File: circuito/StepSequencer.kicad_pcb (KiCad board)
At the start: 2 copper layers, 147.8 x 117.1 mm, 81 parts, among them P1 BEAGLEBONE_BLACK, SW0 SW_PUSH, SW1 SW_PUSH, SW10 SW_PUSH, SW11 SW_PUSH, SW12 SW_PUSH, SW13 SW_PUSH, SW14 SW_PUSH, SW15 SW_PUSH, SW2 SW_PUSH, SW3 SW_PUSH, SW4 SW_PUSH, SW5 SW_PUSH, SW6 SW_PUSH, SW7 SW_PUSH, SW8 SW_PUSH, SW9 SW_PUSH

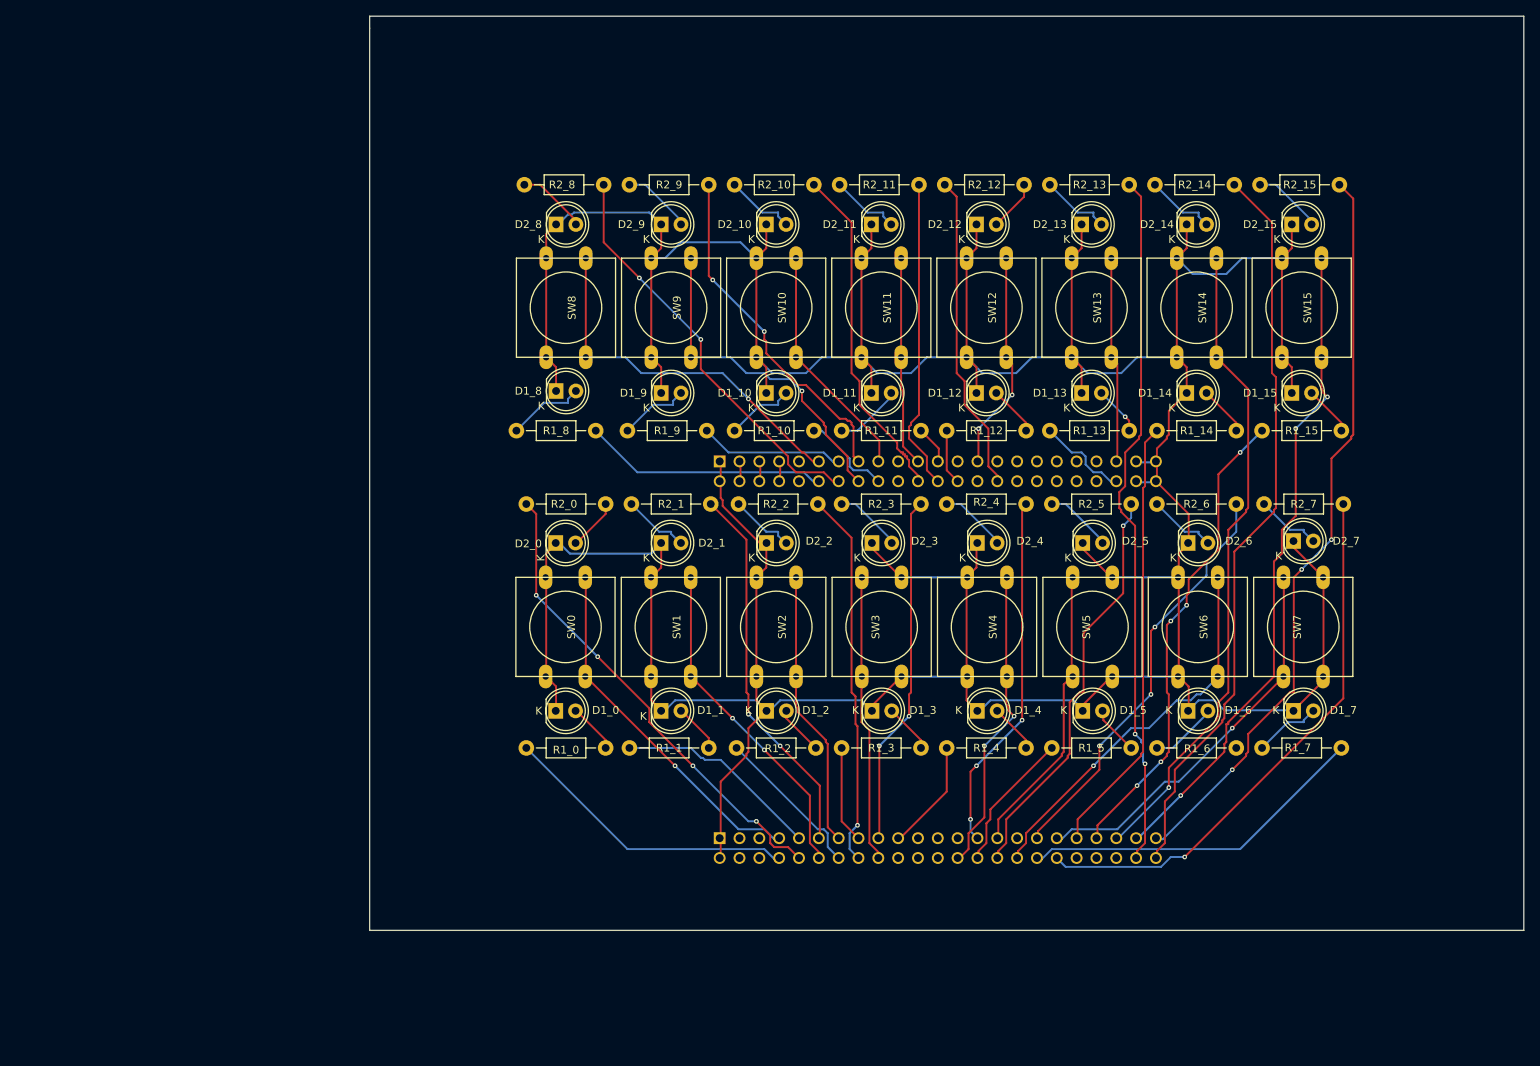
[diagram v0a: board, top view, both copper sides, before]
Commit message: PCB Casi listo
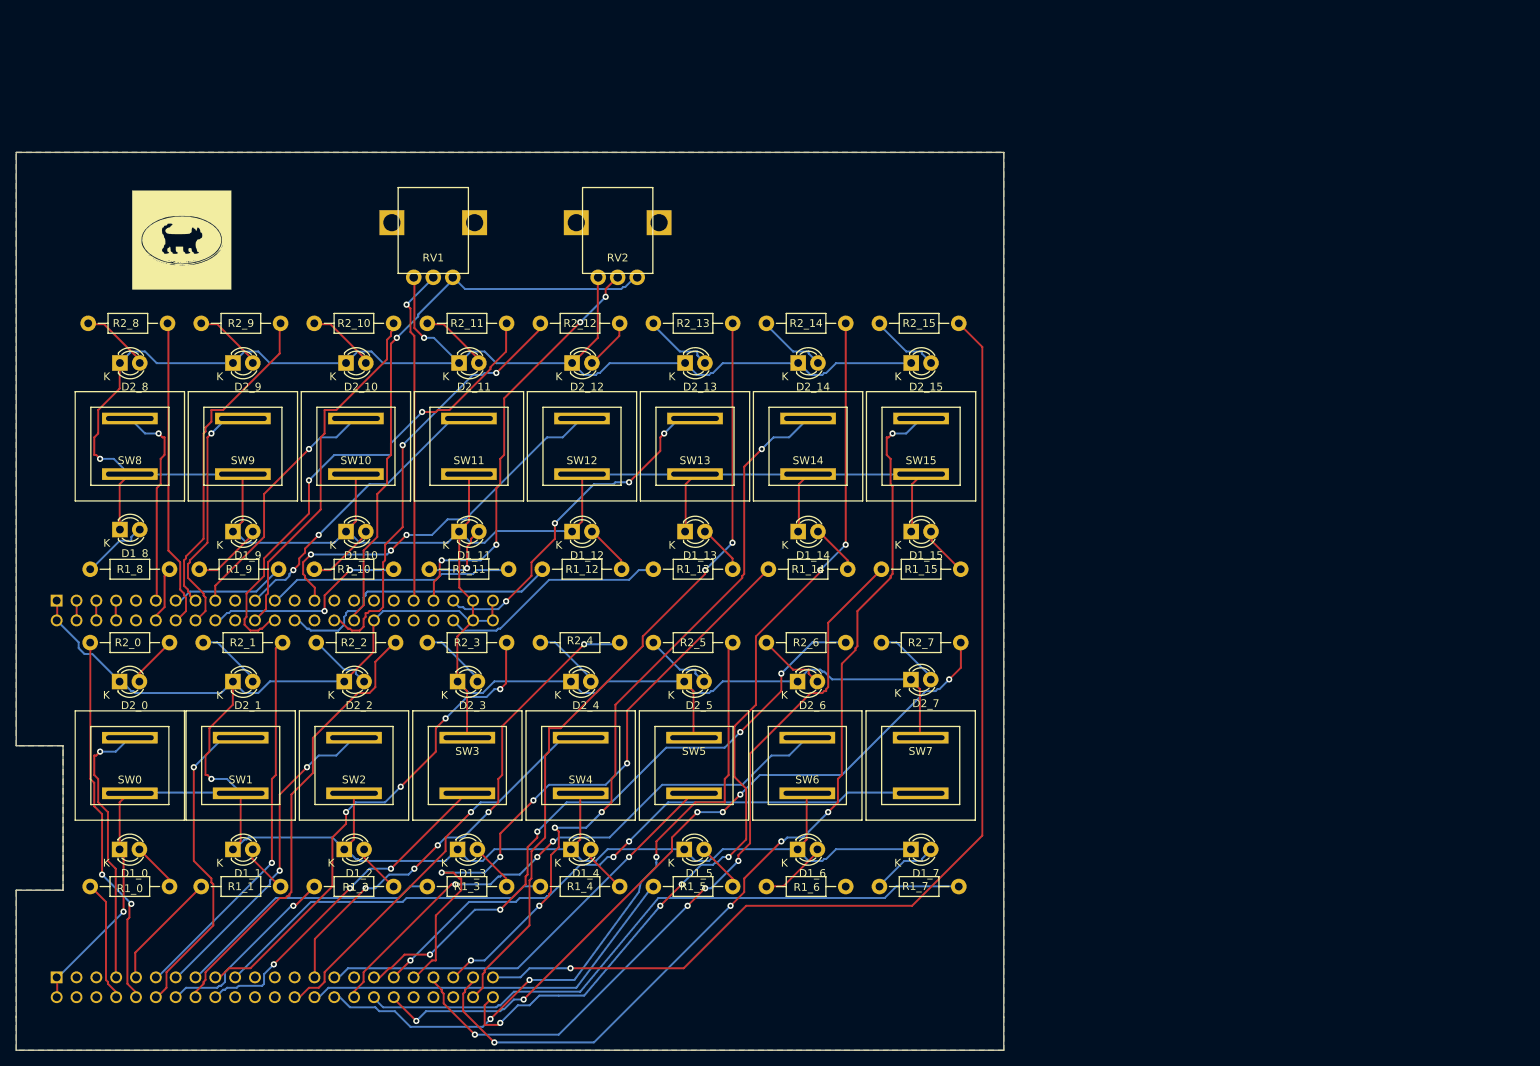
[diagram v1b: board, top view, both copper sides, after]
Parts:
- added ?: , StepSequencer:LOGO, F.Cu at (104.5, 48.0)
- added RV1: POT, StepSequencer:POT_AZUL, F.Cu at (136.7, 52.8)
- added RV2: POT, StepSequencer:POT_AZUL, F.Cu at (160.3, 52.8)
- D1_0, D1_1, D1_10, D1_11, D1_12, D1_13, D1_14, D1_15, D1_2, D1_3, D1_4, D1_5, D1_6, D1_7, D1_8, D1_9, D2_0, D2_1, D2_10, D2_11, D2_12, D2_13, D2_14, D2_15, D2_2, D2_3, D2_4, D2_5, D2_6, D2_7, D2_8, D2_9: footprint LEDs:LED-5MM -> LEDs:LED-3MM
- SW0, SW1, SW10, SW11, SW12, SW13, SW14, SW15, SW2, SW3, SW4, SW5, SW6, SW7, SW8, SW9: footprint Buttons_Switches_ThroughHole:SW_PUSH-12mm -> StepSequencer:BOTON
- moved P1 86.8 mm to (68.8, 92.2)
- moved D1_0 58.6 mm to (96.5, 126.0)
- moved D1_8 58.6 mm to (96.5, 85.1)
- moved D2_0 58.6 mm to (96.5, 104.5)
- moved D2_8 58.6 mm to (96.5, 63.7)
- moved R2_8 58.6 mm to (97.6, 58.6)
- moved R1_0 58.6 mm to (97.8, 130.8)
- moved R2_0 58.6 mm to (97.8, 99.5)
- moved SW8 58.6 mm to (97.8, 74.4), turned to 0 degrees
- moved SW0 58.6 mm to (97.8, 115.3), turned to 0 degrees
- moved SW1 57.9 mm to (112.0, 115.3), turned to 0 degrees
- moved D1_1 57.6 mm to (111.0, 126.0)
- moved D2_1 57.6 mm to (111.0, 104.5)
- moved R2_1 57.6 mm to (112.3, 99.5)
- moved SW9 57.6 mm to (112.3, 74.4), turned to 0 degrees
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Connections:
- P1 pad B34: GNDA -> GNDD
- P1 pad B37: (no net) -> /pot0
- P1 pad B39: (no net) -> /pot1
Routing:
- net GNDD: track 623.7 -> 700.0 mm, vias 0 -> 4
- net +1V8: track 0.00 -> 74.3 mm, vias 0 -> 1
- net /pot1: track 0.00 -> 54.3 mm, vias 0 -> 4
- net /pot0: track 0.00 -> 43.6 mm, vias 0 -> 1
- net /led2_15: track 95.9 -> 137.1 mm, vias 3 -> 1
- net /btn15: track 85.0 -> 123.9 mm, vias 3 -> 5
- net /led1_7: track 44.9 -> 82.7 mm
- net /led1_15: track 61.4 -> 98.5 mm, vias 5 -> 4
- net /led2_5: track 53.0 -> 87.9 mm, vias 1 -> 3
- net /led1_5: track 18.3 -> 50.4 mm
- net /led1_4: track 14.3 -> 44.3 mm
- net /led1_12: track 7.06 -> 37.1 mm
- net /led2_6: track 53.6 -> 82.9 mm, vias 3 -> 5
- net /btn7: track 50.6 -> 77.6 mm, vias 1 -> 3
- net /led1_11: track 5.19 -> 31.7 mm
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- added copper zone on B.Cu, net GNDD
- added copper zone on F.Cu, net GNDD
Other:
- board size 147.8 x 117.1 mm -> 126.5 x 115 mm
- net class Default: via_dia 0.6 -> 0.8
